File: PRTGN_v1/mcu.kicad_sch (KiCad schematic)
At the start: 15 parts, among them U1 ESP32-S3-WROOM-1

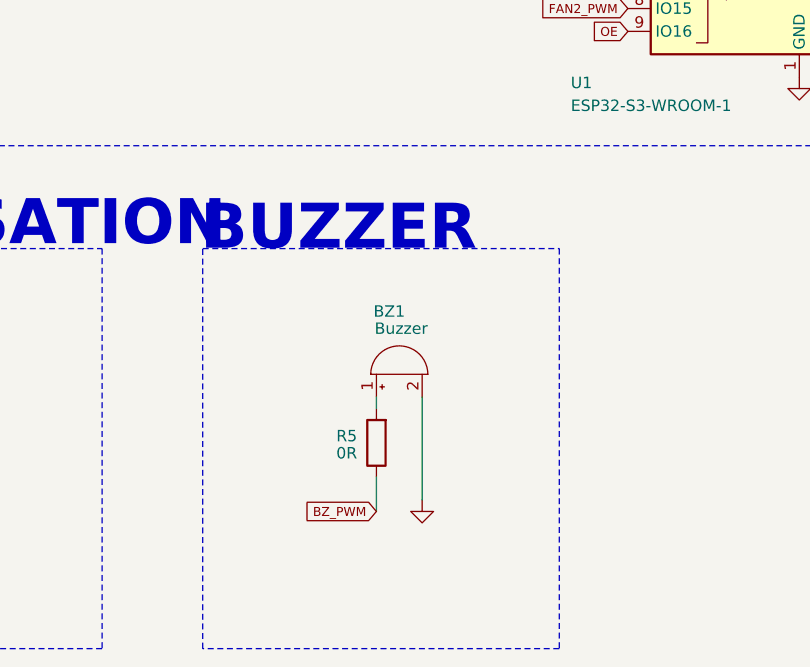
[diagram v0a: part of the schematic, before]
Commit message: pcb updates
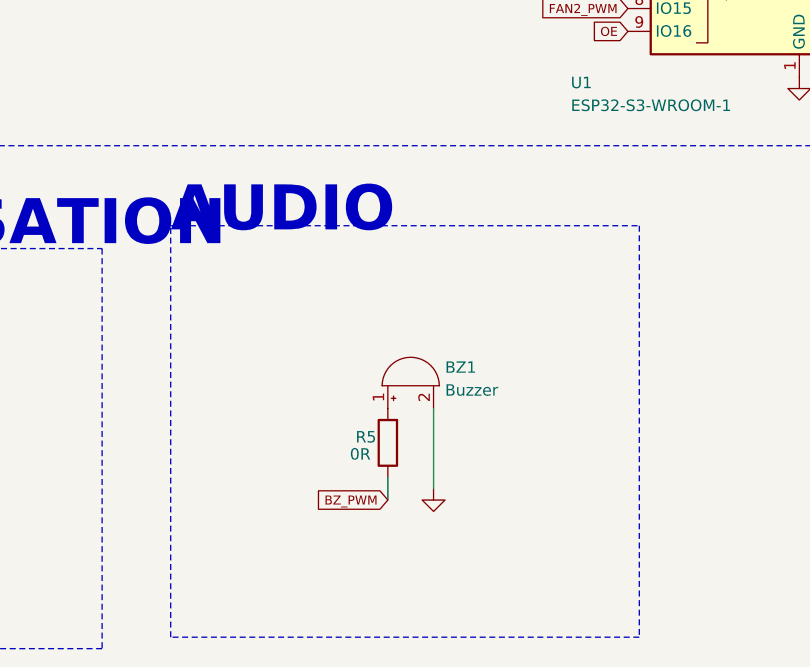
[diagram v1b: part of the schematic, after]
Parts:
- BZ1: footprint Schrack_brd:BUZZER_CUI_CPT -> gps-compass_brd:CEM-1203_Buzzer
- R5: footprint Resistor_SMD:R_0805_2012Metric_Pad1.20x1.40mm_HandSolder -> Resistor_SMD:R_0805_2012Metric; LCSC (none) -> C17633
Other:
- note added: "AUDIO"
- note removed: "BUZZER"
